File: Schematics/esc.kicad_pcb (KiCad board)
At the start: 4 copper layers, 62.5 x 38 mm, 79 parts, among them IC1 74HCT08BQ,115, IC2 74HCT08BQ,115, J1 8730, J10 AVR-ISP-10, J11 Conn_01x06, J2 8730, J3 8730, J4 8730, J5 8730, J6 Conn_01x01, J7 Conn_01x01, J8 Conn_01x01, J9 Conn_01x06, U1 TLV76750DRVx, U2 ATmega328P-M, U3 DRV8300DRGER

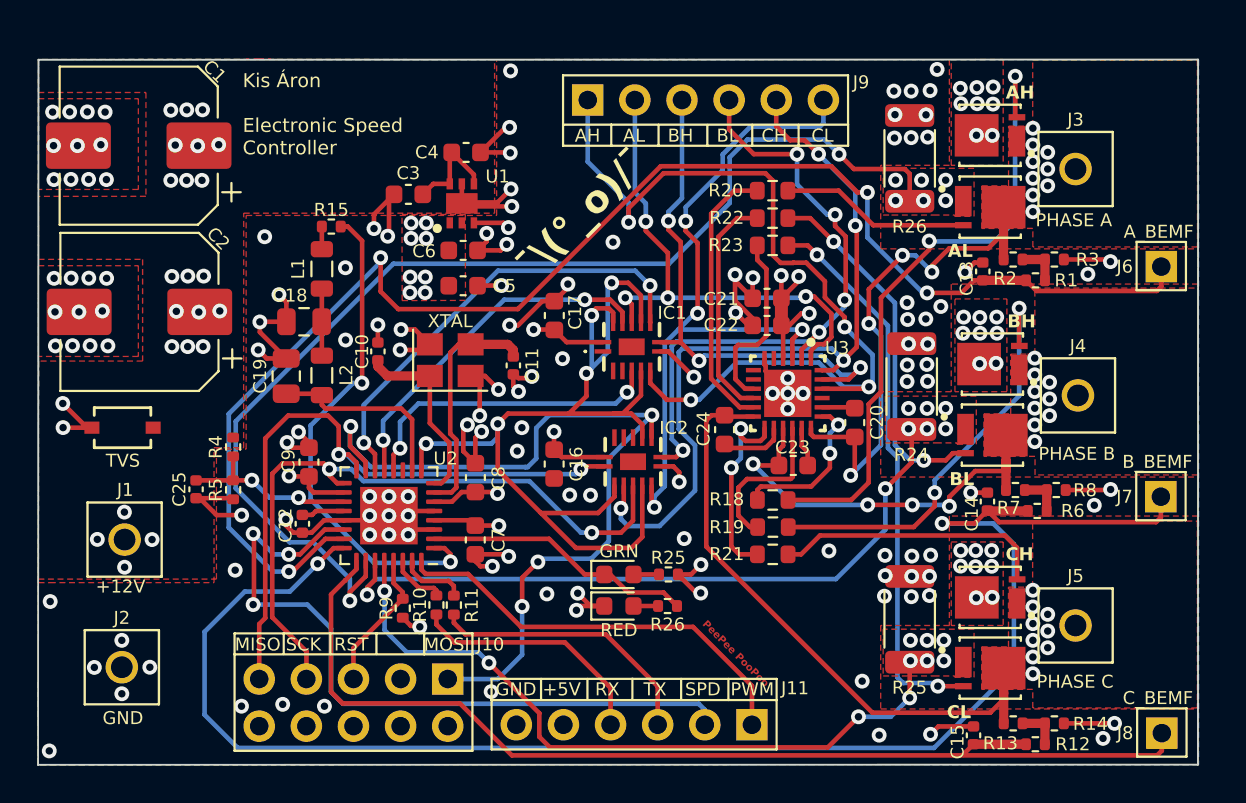
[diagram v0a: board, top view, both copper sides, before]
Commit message: V1.0
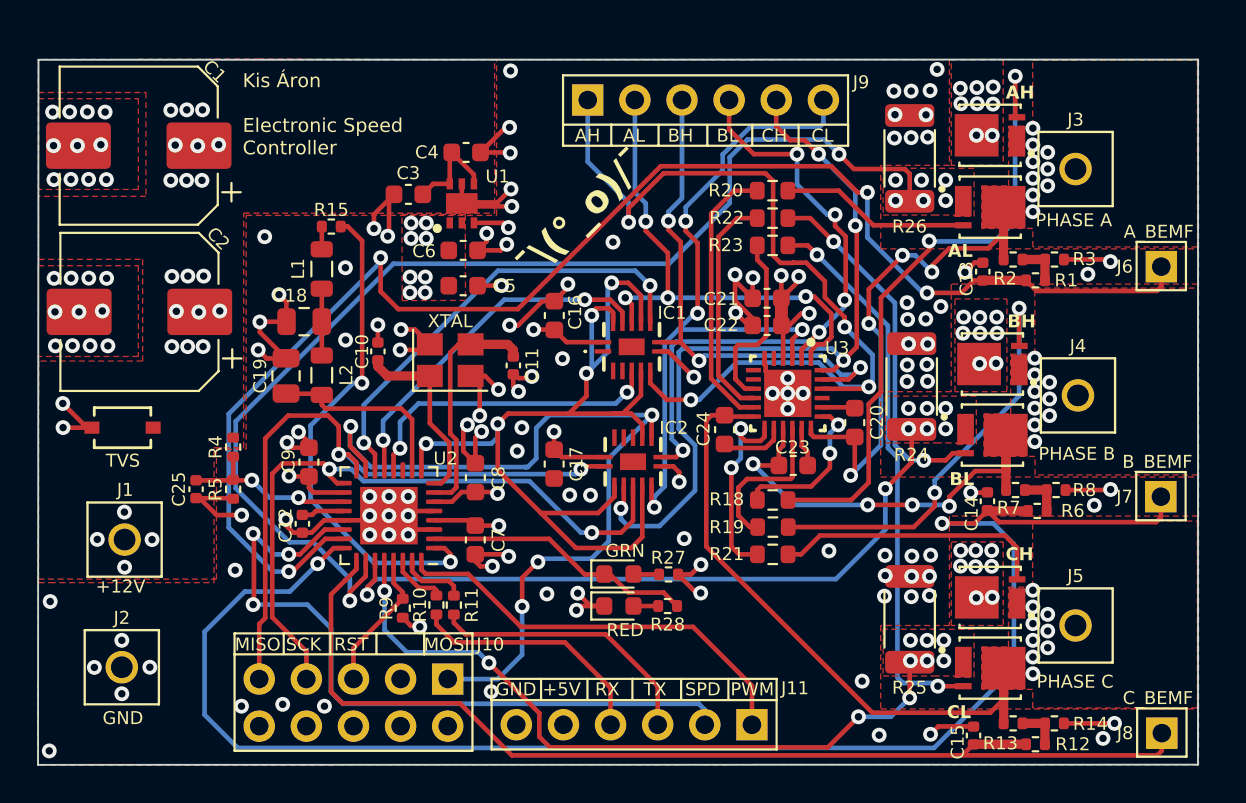
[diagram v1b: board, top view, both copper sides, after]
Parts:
- removed the R25 at (80.0, 59.8)
- removed the R26 at (79.9, 61.5)
- added R27: 300, Resistor_SMD:R_0402_1005Metric, F.Cu at (80.0, 59.8)
- added R28: 300, Resistor_SMD:R_0402_1005Metric, F.Cu at (79.9, 61.5)
- C13, C14, C15: value 2.4n -> 2.2n
- R14, R3, R8: value 10k -> 20k
- R5: value 10k -> 7.5k
- turned L1 to 90 degrees
- turned R13 to 0 degrees
- turned R7 to 0 degrees
- turned R12 to 0 degrees
- turned R1 to 0 degrees
- turned R2 to 0 degrees
- turned R6 to 0 degrees
- renumbered C17 to C16, C16 to C17
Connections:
- R1 pad 1: Net-(R1-Pad1) -> COIL_A_BEMF
- R1 pad 2: COIL_A_BEMF -> Net-(R1-Pad2)
- R12 pad 1: Net-(R12-Pad1) -> COIL_C_BEMF
- R12 pad 2: COIL_C_BEMF -> Net-(R12-Pad2)
- R13 pad 1: Net-(R12-Pad1) -> COIL_C
- R13 pad 2: COIL_C -> Net-(R12-Pad2)
- R14 pad 2: Net-(R12-Pad1) -> Net-(R12-Pad2)
- R2 pad 1: Net-(R1-Pad1) -> COIL_A
- R2 pad 2: COIL_A -> Net-(R1-Pad2)
- R3 pad 2: Net-(R1-Pad1) -> Net-(R1-Pad2)
- R6 pad 1: Net-(R6-Pad1) -> COIL_B_BEMF
- R6 pad 2: COIL_B_BEMF -> Net-(R6-Pad2)
- R7 pad 1: Net-(R6-Pad1) -> COIL_B
- R7 pad 2: COIL_B -> Net-(R6-Pad2)
- R8 pad 2: Net-(R6-Pad1) -> Net-(R6-Pad2)
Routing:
- net Net-(GRN1-A): track 1.38 -> 4.48 mm, vias 0 -> 2
- net +5V: track 23.0 -> 19.9 mm, vias 16 -> 14
- net Net-(R1-Pad2): track 0.00 -> 2.33 mm
- net Net-(R1-Pad1): track 2.33 -> 0.00 mm
- net Net-(R12-Pad2): track 0.00 -> 2.33 mm
- net Net-(R12-Pad1): track 2.33 -> 0.00 mm
- net Net-(R6-Pad2): track 0.00 -> 2.31 mm
- net Net-(R6-Pad1): track 2.31 -> 0.00 mm
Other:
- board text removed: "PeePee PooPoo"
